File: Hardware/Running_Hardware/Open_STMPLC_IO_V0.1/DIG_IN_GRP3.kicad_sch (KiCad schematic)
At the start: 54 parts, among them J27 Screw_Terminal_01x02, J28 Screw_Terminal_01x02, J29 Screw_Terminal_01x02, J30 Screw_Terminal_01x02, J31 Screw_Terminal_01x02, J32 Screw_Terminal_01x02, U31 6N137, U32 6N137, U33 6N137, U34 6N137, U35 6N137, U36 6N137

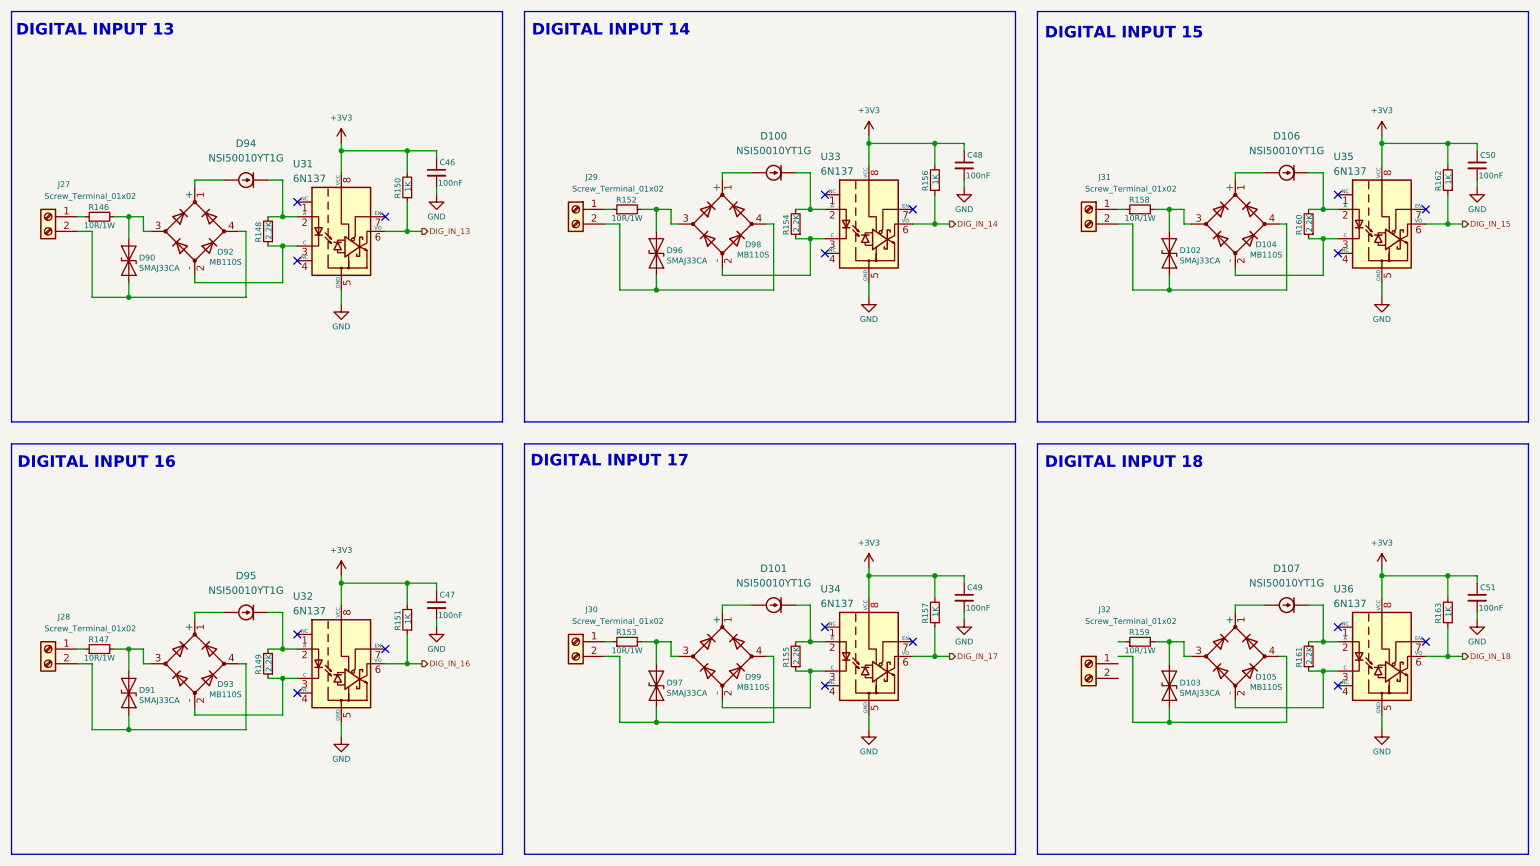
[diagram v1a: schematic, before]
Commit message: Analog input section
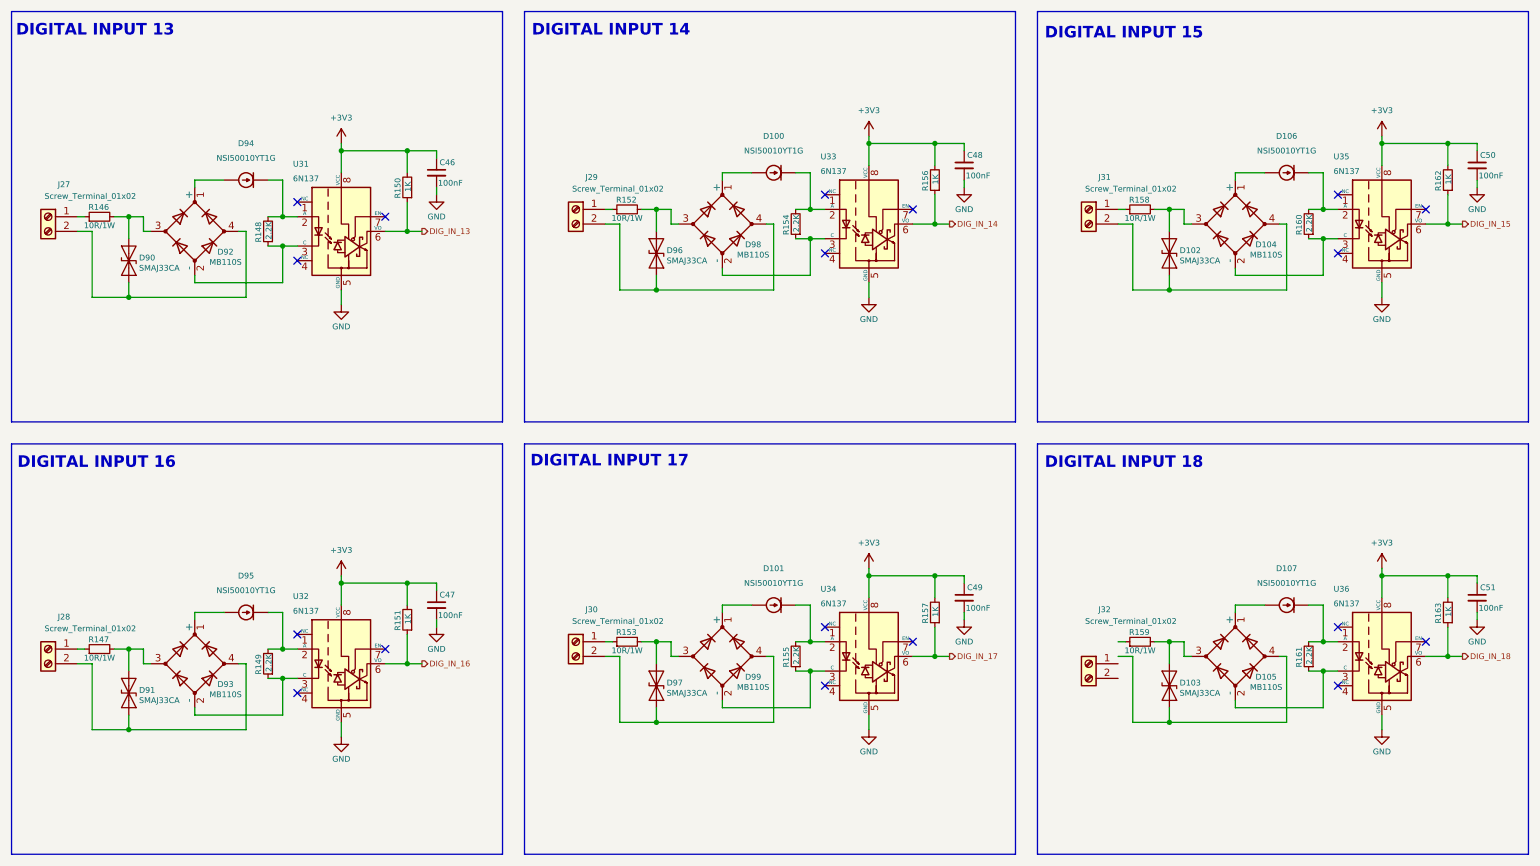
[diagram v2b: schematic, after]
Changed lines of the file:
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@@
 			(effects
 				(font
-					(size 1.27 1.27)
+					(size 1 1)
 				)
 				(justify left)
@@
 			(effects
 				(font
-					(size 1.27 1.27)
+					(size 1 1)
 				)
 				(justify left)
@@
 			(effects
 				(font
-					(size 1.27 1.27)
+					(size 1 1)
 				)
 			)
@@
 			(effects
 				(font
-					(size 1.27 1.27)
+					(size 1 1)
 				)
 			)
@@
 			(effects
 				(font
-					(size 1.27 1.27)
+					(size 1 1)
 				)
 			)
@@
 			(effects
 				(font
-					(size 1.27 1.27)
+					(size 1 1)
 				)
 			)
@@
 			(effects
 				(font
-					(size 1.27 1.27)
+					(size 1 1)
 				)
 			)
@@
 			(effects
 				(font
-					(size 1.27 1.27)
+					(size 1 1)
 				)
 			)
@@
 			(effects
 				(font
-					(size 1.27 1.27)
+					(size 1 1)
 				)
 				(justify left)
@@
 			(effects
 				(font
-					(size 1.27 1.27)
+					(size 1 1)
 				)
 				(justify left)
@@
 			(effects
 				(font
-					(size 1.27 1.27)
+					(size 1 1)
 				)
 			)
@@
 			(effects
 				(font
-					(size 1.27 1.27)
+					(size 1 1)
 				)
 			)
@@
 			(effects
 				(font
-					(size 1.27 1.27)
+					(size 1 1)
 				)
 				(justify left)
@@
 			(effects
 				(font
-					(size 1.27 1.27)
+					(size 1 1)
 				)
 				(justify left)
@@
 			(effects
 				(font
-					(size 1.27 1.27)
+					(size 1 1)
 				)
 				(justify left)
@@
 			(effects
 				(font
-					(size 1.27 1.27)
+					(size 1 1)
 				)
 				(justify left)
@@
 			(effects
 				(font
-					(size 1.27 1.27)
+					(size 1 1)
 				)
 				(justify left)
@@
 			(effects
 				(font
-					(size 1.27 1.27)
+					(size 1 1)
 				)
 				(justify left)
@@
 			(effects
 				(font
-					(size 1.27 1.27)
+					(size 1 1)
 				)
 			)
@@
 			(effects
 				(font
-					(size 1.27 1.27)
+					(size 1 1)
 				)
 			)
@@
 			(effects
 				(font
-					(size 1.27 1.27)
+					(size 1 1)
 				)
 				(justify left)
@@
 			(effects
 				(font
-					(size 1.27 1.27)
+					(size 1 1)
 				)
 				(justify left)
@@
 			(effects
 				(font
-					(size 1.27 1.27)
+					(size 1 1)
 				)
 			)
@@
 			(effects
 				(font
-					(size 1.27 1.27)
+					(size 1 1)
 				)
 			)
